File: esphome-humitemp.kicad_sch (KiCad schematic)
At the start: 16 parts, among them J1 eflashy32, J2 USB_IN, J3 USB_OUT, U1 SHT35-DISB, U2 TLV75533PDBV, U3 ESP32-WROOM-32D

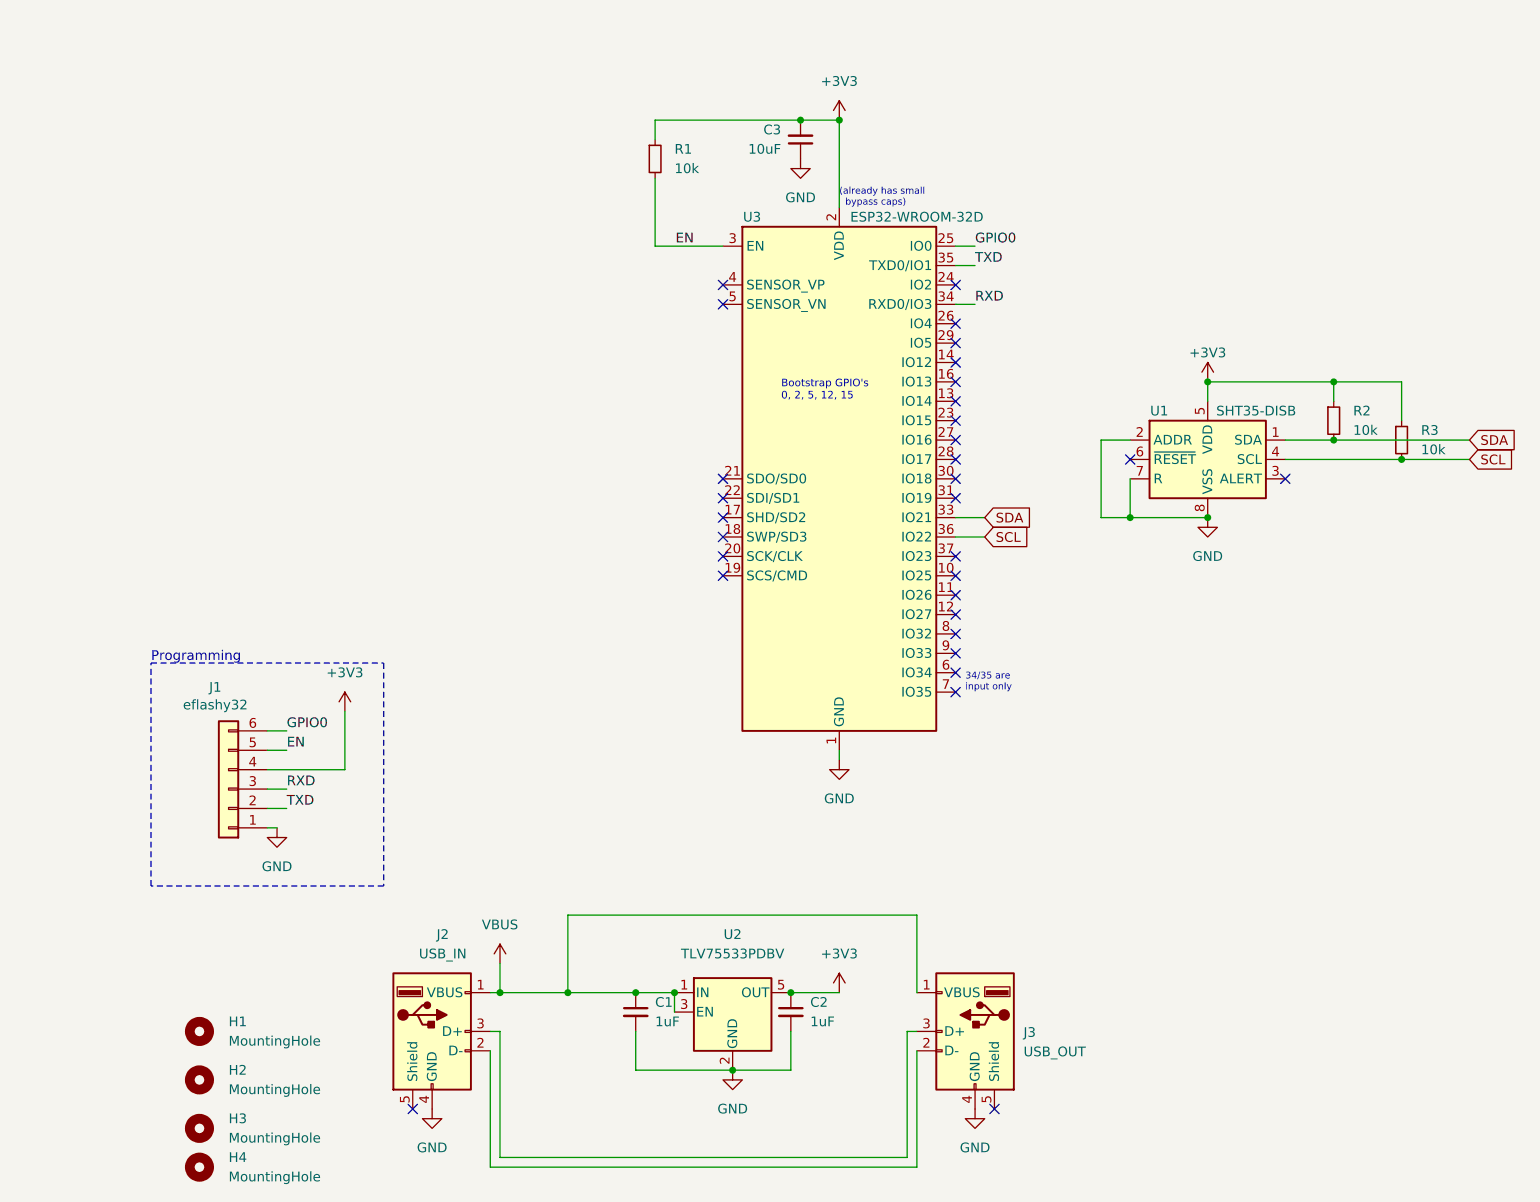
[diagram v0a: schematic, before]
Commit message: v2 ecad
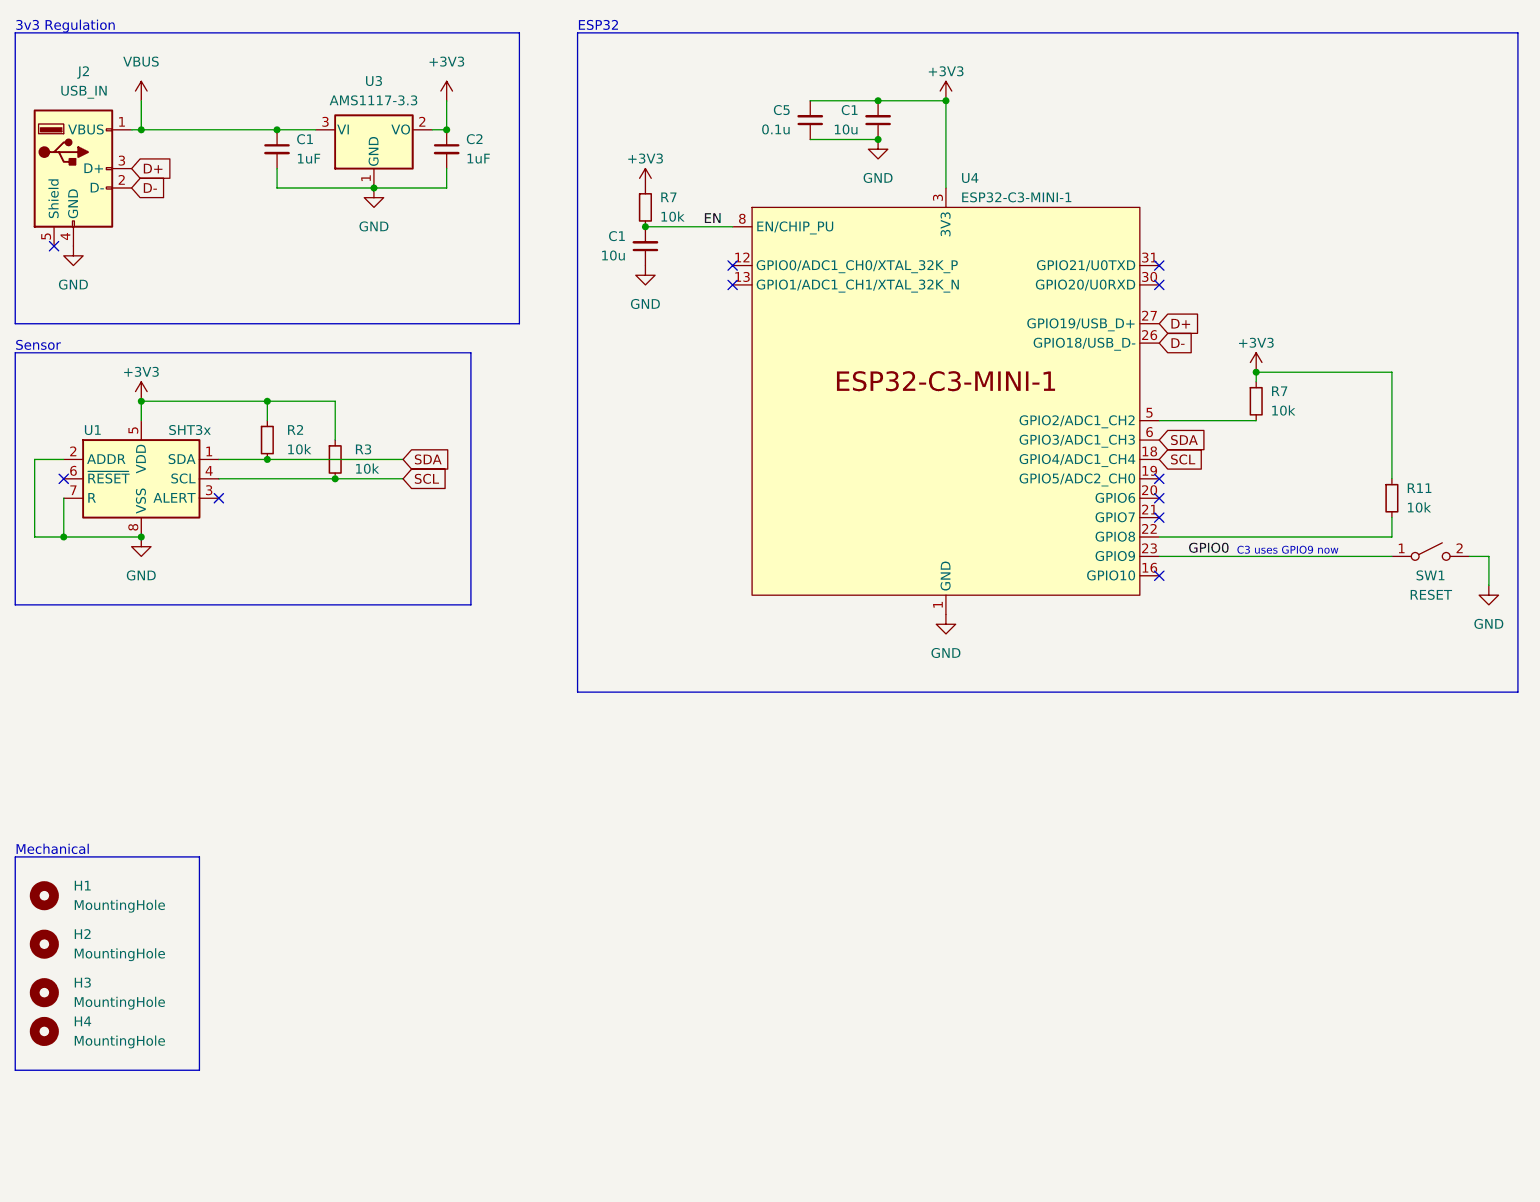
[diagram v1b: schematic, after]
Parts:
- removed C3: 10uF, Capacitor_SMD:C_0805_2012Metric, symbol Device:C_Small
- removed J1: eflashy32, Connector_PinHeader_2.54mm:PinHeader_1x06_P2.54mm_Vertical, symbol Connector_Generic:Conn_01x06
- removed J3: USB_OUT, Connector_USB:USB_A_Molex_67643_Horizontal, symbol Connector:USB_A
- removed R1: 10k, Resistor_SMD:R_0805_2012Metric, symbol Device:R_Small
- removed U2: TLV75533PDBV, Package_TO_SOT_SMD:SOT-23-5, symbol Regulator_Linear:TLV75533PDBV
- removed U3: ESP32-WROOM-32D, RF_Module:ESP32-WROOM-32, symbol RF_Module:ESP32-WROOM-32D
- added C1 (x2): 10u, Capacitor_SMD:C_0805_2012Metric, symbol Device:C_Small
- added C5: 0.1u, Capacitor_SMD:C_0603_1608Metric, symbol Device:C_Small
- added R11, R7 (x2): 10k, Resistor_SMD:R_0402_1005Metric, symbol Device:R_Small
- added SW1: RESET, Button_Switch_SMD:SW_Push_1P1T_XKB_TS-1187A, symbol Switch:SW_SPST
- added U3: AMS1117-3.3, Package_TO_SOT_SMD:SOT-223-3_TabPin2, symbol Regulator_Linear:AP1117-33
- added U4: ESP32-C3-MINI-1, Espressif:ESP32-C3-MINI-1, symbol Espressif:ESP32-C3-MINI-1
- R2, R3: footprint Resistor_SMD:R_0805_2012Metric -> Resistor_SMD:R_0402_1005Metric
- U1: value SHT35-DISB -> SHT3x; LCSC C90161 -> C80862
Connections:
- net +3V3: now also C1.2, C5.2, R11.1, R7.1, R7.1, U3.2 (VO), U4.3 (3V3)
- net EN: now also C1.2, R7.2, U4.8 (EN/CHIP_PU)
- net GND: now also C1.1, C1.1, C5.1, SW1.2 (B), U3.1 (GND), U4.1 (GND), U4.11 (GND), U4.14 (GND), U4.2 (GND), U4.36 (GND), U4.37 (GND), U4.38 (GND), U4.39 (GND), U4.40 (GND), U4.41 (GND), U4.42 (GND), U4.43 (GND), U4.44 (GND), U4.45 (GND), U4.46 (GND), U4.47 (GND), U4.48 (GND), U4.49 (GND), U4.50 (GND), U4.51 (GND), U4.52 (GND), U4.53 (GND)
- net GPIO0: now also SW1.1 (A), U4.23 (GPIO9)
- net SCL: now also U4.18 (GPIO4/ADC1_CH4)
- net SDA: now also U4.6 (GPIO3/ADC1_CH3)
- net VBUS: now also U3.3 (VI)
- net D-: now reaches J2.2 (D-)
- net D-: now also U4.26 (GPIO18/USB_D-)
- net D+: now reaches J2.3 (D+)
- net D+: now also U4.27 (GPIO19/USB_D+)
- new net: R7.2, U4.5 (GPIO2/ADC1_CH2)
- new net: R11.2, U4.22 (GPIO8)
- no-connect marks 31 -> 11
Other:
- note added: "3v3 Regulation"
- note added: "C3 uses GPIO9 now"
- note added: "ESP32"
- note added: "Mechanical"
- note added: "Sensor"
- note removed: "(already has small bypass caps)"
- note removed: "34/35 are input only"
- note removed: "Bootstrap GPIO's 0, 2, 5, 12, 15"
- note removed: "Programming"
- moved on the sheet: C1, C2, H1, H2, H3, H4, J2, R2, R3, U1
